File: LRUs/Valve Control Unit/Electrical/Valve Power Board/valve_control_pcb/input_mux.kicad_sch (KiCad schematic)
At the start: 24 parts, among them Q17 SiR882ADP, Q18 SiR882ADP, Q21 SiR882ADP, Q22 SiR882ADP, Q5 AO3400A, Q6 AO3400A, U5 LTC4359-MS8, U6 LTC4359-MS8

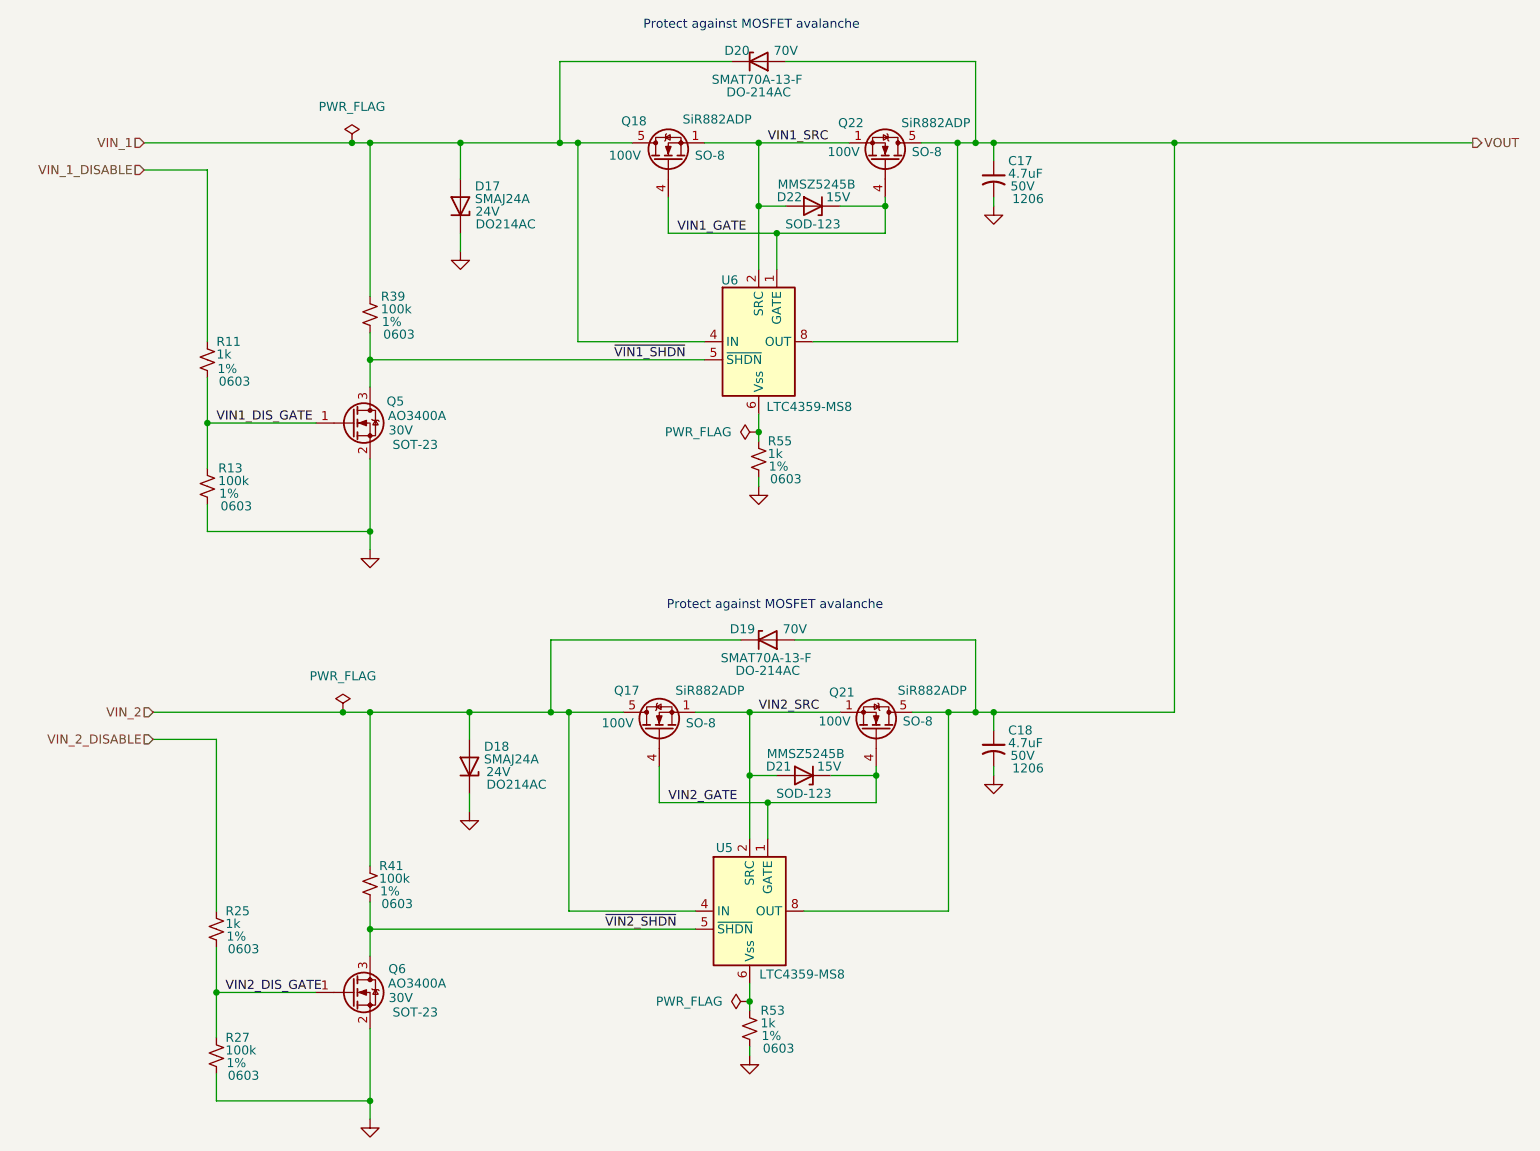
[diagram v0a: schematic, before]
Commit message: Major changes
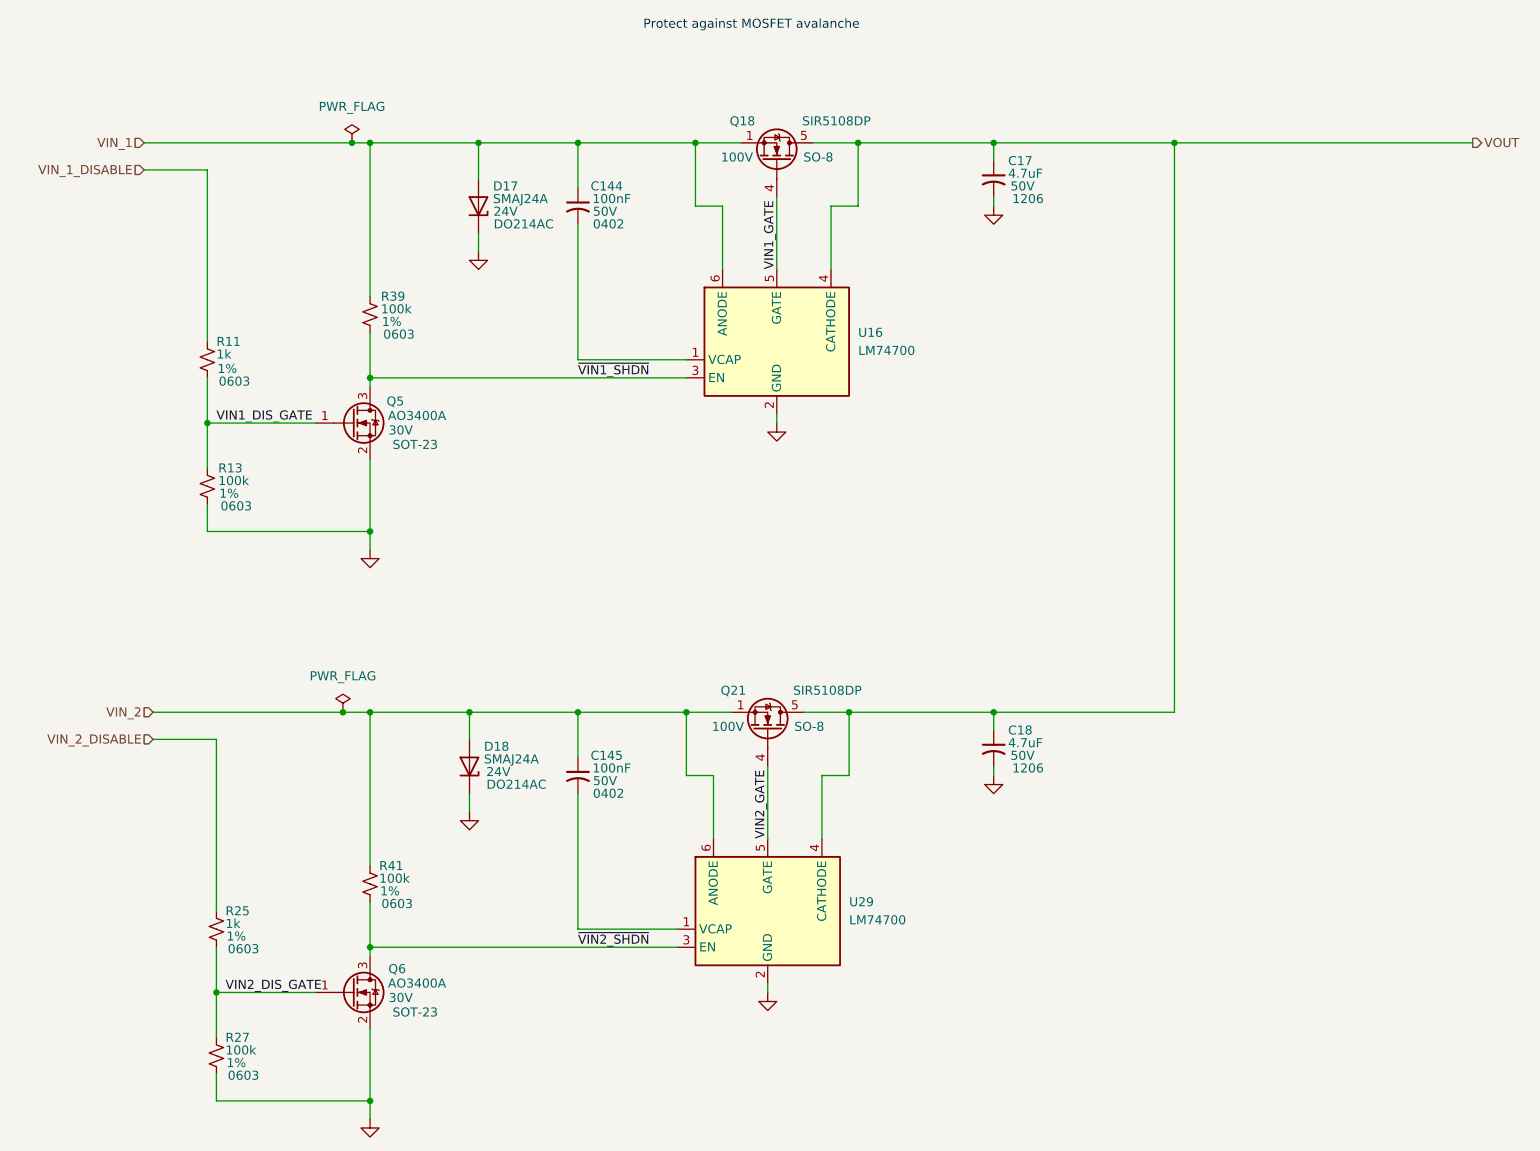
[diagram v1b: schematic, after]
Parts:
- removed D19, D20: SMAT70A-13-F, Diode_SMD:D_SMA, symbol Device:D_Zener
- removed D21, D22: MMSZ5245B, Diode_SMD:D_SOD-123, symbol Device:D_Zener
- removed Q17, Q22: SiR882ADP, Package_SO:PowerPAK_SO-8_Single, symbol Transistor_FET:SiR696DP
- removed R53, R55: 1k, valve_pcb_footprints:R_0603_1608Metric, symbol Device:R_Small_US
- removed U5, U6: LTC4359-MS8, Package_SO:MSOP-8_3x3mm_P0.65mm, symbol Power_Management:LTC4359-MS8
- added C144, C145: 100nF, valve_pcb_footprints:C_0402_1005Metric, symbol Device:C_Small_US
- added U16, U29: LM74700, Package_TO_SOT_SMD:SOT-23-6_Handsoldering, symbol Power_Management:LM74700
- Q18, Q21: value SiR882ADP -> SIR5108DP; footprint Package_SO:PowerPAK_SO-8_Single -> valve_pcb_footprints:PowerPAK_SO-8_Single; JLCPCB Part # C553986 -> C53262900
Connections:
- net VIN1_SRC is gone; now on net VIN_1: Q18.1 (S), Q18.2 (S), Q18.3 (S)
- net VIN2_SRC is gone; now on net VIN_2: Q21.1 (S), Q21.2 (S), Q21.3 (S)
- net GND: now also U16.2 (GND), U29.2 (GND)
- net VIN1_GATE: now also U16.5 (GATE)
- net VIN2_GATE: now also U29.5 (GATE)
- net VIN_1: now also C144.1, U16.6 (ANODE); no longer Q18.5 (D)
- net VIN_2: now also C145.1, U29.6 (ANODE)
- net VOUT: now also Q18.5 (D), U16.4 (CATHODE), U29.4 (CATHODE)
- net ~{VIN1_SHDN}: now also U16.3 (EN)
- net ~{VIN2_SHDN}: now also U29.3 (EN)
- new net: C144.2, U16.1 (VCAP)
- new net: C145.2, U29.1 (VCAP)
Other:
- title: (none) -> INPUT MUX
- moved on the sheet: D17
